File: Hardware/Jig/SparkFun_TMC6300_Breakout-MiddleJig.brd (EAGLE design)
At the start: 15.2 x 20.3 mm, 57 parts, among them U2 TMC6300

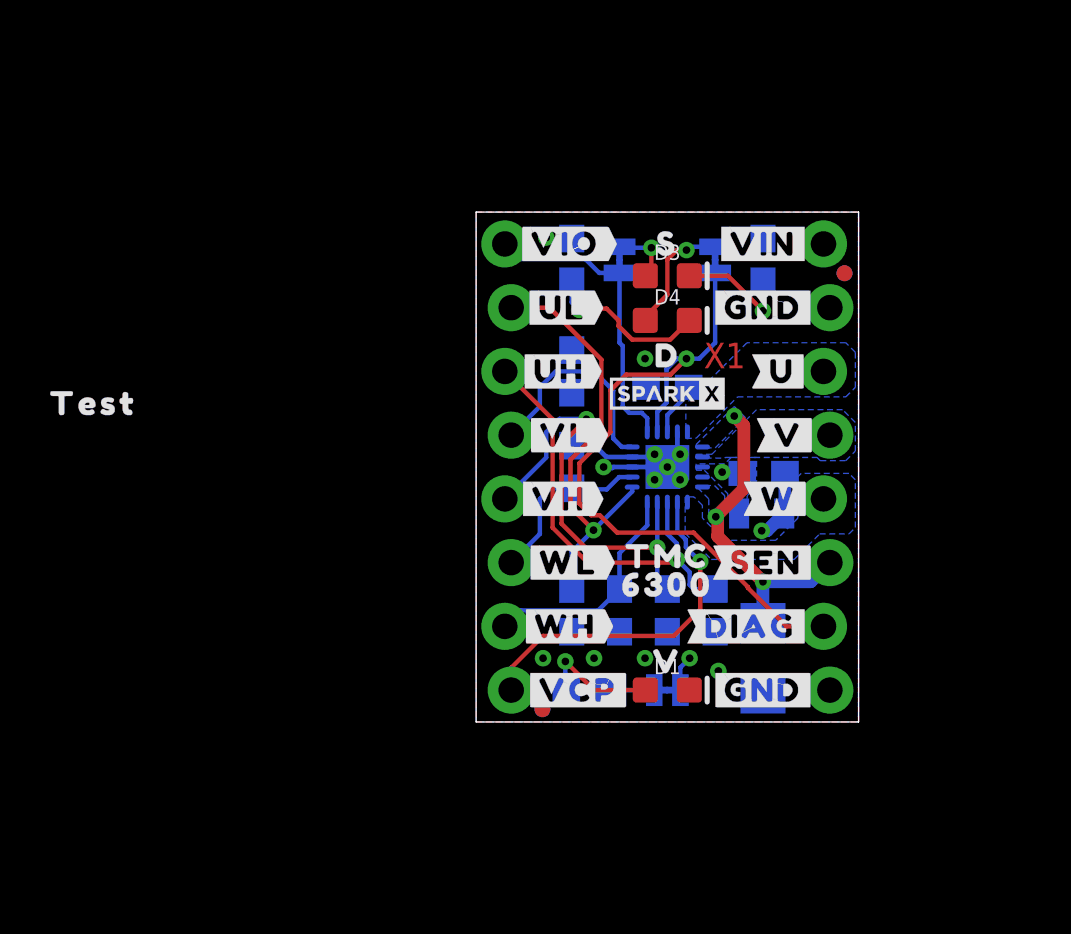
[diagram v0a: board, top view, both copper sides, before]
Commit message: Add production files
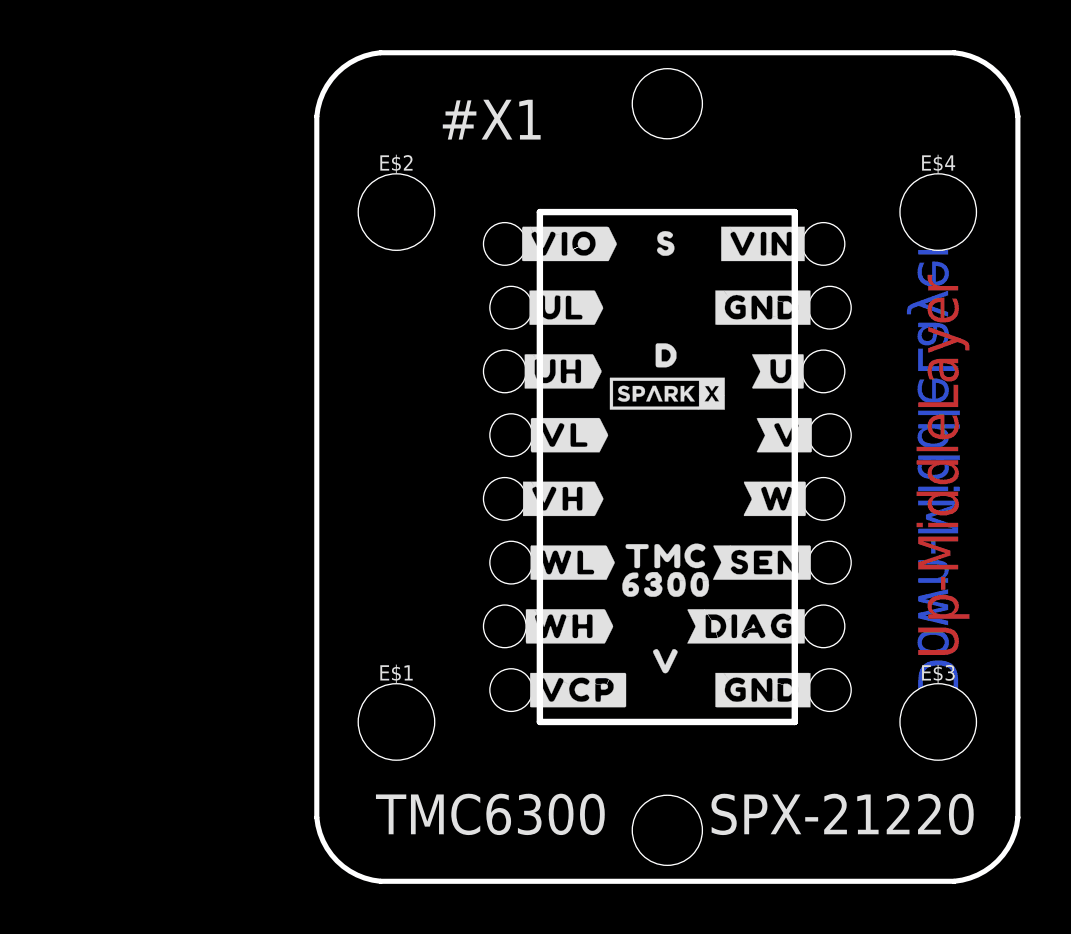
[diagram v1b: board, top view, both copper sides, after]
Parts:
- removed C3: 10uF, SparkFun-Capacitors:0805
- removed C4, C5: 0.1uF, SparkFun-Capacitors:0603
- removed D, S, V: JUMPER-SMT_2_NC_TRACE_SILK, SparkFun-Jumpers:SMT-JUMPER_2_NC_TRACE_SILK
- removed D1: RED, SparkFun-LED:LED-0603
- removed D3: BLUE, SparkFun-LED:LED-0603
- removed D4: GREEN, SparkFun-LED:LED-0603
- removed FD1, FD2, FD3, FD4: FIDUCIALUFIDUCIAL, SparkFun-Aesthetics:FIDUCIAL-MICRO
- removed J1, J2: (no value), SparkFun-Connectors:1X08_LOCK_NO_SILK
- removed R10, R5, R6, R7, R8, R9: 100k, SparkFun-Resistors:0603
- removed R14, R4: 330, SparkFun-Resistors:0603
- removed R15: 0.12, SparkFun-Resistors:1206
- removed R3: 1k, SparkFun-Resistors:0603
- removed U$4: (no value), output:TEST0
- removed U2: TMC6300, TMC6300:QFN-20
- added E$1, E$2, E$3, E$4: (no value), SparkFun-Hardware:STAND-OFF-TIGHT
- added E$5, E$6: (no value), SparkFun-Hardware:NUBBIN_LOCKER
- moved LOGO2 47.0 mm to (43.2, 50.8)
- moved FRAME1 47.0 mm to (73.7, -11.4)
- moved LOGO1 47.0 mm to (59.7, -2.54)
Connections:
- removed net DIAG: D.2, J2.7, U2.12
- removed net GND: C3.2, C4.2, C5.2, D1.C, J2.2, J2.8, R10.1, R14.1, R15.1, R4.1, R5.1, R6.1, R7.1, R8.1, R9.1, U2.14, U2.8, U2.9, U2.PAD
- removed net N$1: R3.2, V.1
- removed net N$10: D3.C, R4.2
- removed net N$12: D4.C, R14.2
- removed net N$4: D1.A, R3.1
- removed net N$5: D3.A, S.1
- removed net N$6: C5.1, U2.13
- removed net N$9: D.1, D4.A
- removed net SENSE: J2.6, R15.2, U2.16, U2.20
- removed net U: J2.3, U2.15
- removed net UH: J1.6, R10.2, U2.3
- removed net UL: J1.7, R9.2, U2.6
- removed net V: J2.4, U2.17
- removed net VCP: J1.1, U2.2
- removed net VH: J1.4, R8.2, U2.4
- removed net VIN: C3.1, C4.1, J2.1, U2.18, V.2
- removed net VIO/!STDBY!: J1.8, S.2, U2.11
- removed net VL: J1.5, R7.2, U2.10
- removed net W: J2.5, U2.1
- removed net WH: J1.2, R6.2, U2.5
- removed net WL: J1.3, R5.2, U2.7
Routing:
- net DIAG: track 28.2 -> 0.00 mm, vias 1 -> 0
- net VH: track 17.6 -> 0.00 mm, vias 2 -> 0
- net UH: track 17.3 -> 0.00 mm, vias 1 -> 0
- net UL: track 17.2 -> 0.00 mm, vias 1 -> 0
- net VCP: track 14.0 -> 0.00 mm, vias 1 -> 0
- net SENSE: track 12.6 -> 0.00 mm, vias 3 -> 0
- net VIO/!STDBY!: track 12.2 -> 0.00 mm
- net VL: track 9.53 -> 0.00 mm
- net WH: track 9.11 -> 0.00 mm
- net GND: track 8.12 -> 0.00 mm, vias 13 -> 0
- net WL: track 7.09 -> 0.00 mm
- net N$12: track 6.63 -> 0.00 mm, vias 1 -> 0
- net N$9: track 4.90 -> 0.00 mm, vias 1 -> 0
- net N$4: track 4.82 -> 0.00 mm, vias 1 -> 0
- net N$10: track 4.69 -> 0.00 mm, vias 1 -> 0
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- removed copper zone on layer 1, net GND
- removed copper zone on layer 16, net GND
- removed copper zone on layer 2, net GND
- removed copper zone on layer 16, net SENSE
- removed copper zone on layer 16, net U
- removed copper zone on layer 16, net V
- removed copper zone on layer 15, net VIN
- removed copper zone on layer 16, net VIN
- removed copper zone on layer 16, net W
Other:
- board size 15.2 x 20.3 mm -> 27.9 x 33 mm
- board text added: "#X1"
- board text added: "Down-MiddleLayer"
- board text added: "SPX-21220"
- board text added: "TMC6300"
- board text added: "Up-MiddleLayer"
- board text removed: "X1"
